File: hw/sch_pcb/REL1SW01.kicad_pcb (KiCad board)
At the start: 2 copper layers, 30 x 40.1 mm, 22 parts, among them J1 HEADER_2x02_PARALLEL, J2 HEADER_2x02_PARALLEL, J3 HEADER_2x06_PARALLEL, J4 HEADER_2x06_PARALLEL, J5 HEADER_2x04_PARALLEL, M1 SROUB3M, M2 SROUB3M, M3 SROUB3M, M4 SROUB3M, T1 IRLML6244, T2 IRLML6244, X1 RELE

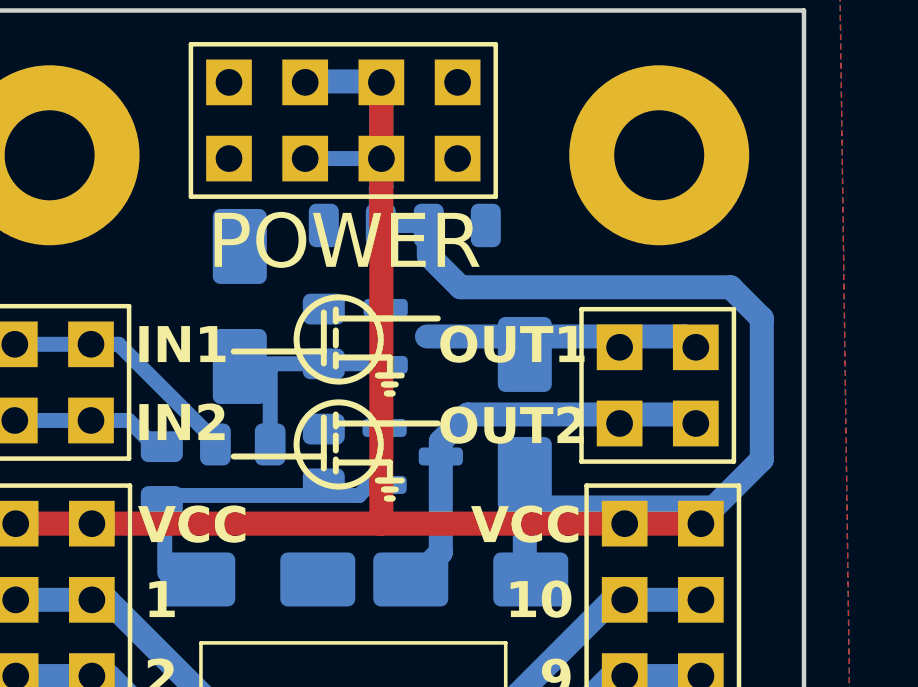
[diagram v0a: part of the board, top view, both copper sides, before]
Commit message: update template
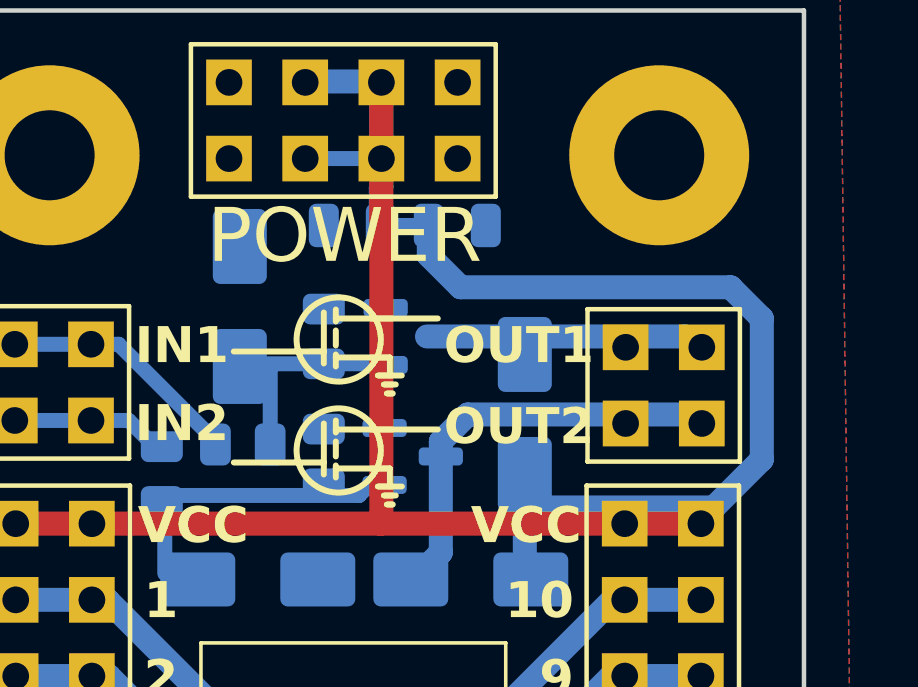
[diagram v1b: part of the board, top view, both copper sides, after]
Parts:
- moved J2 0.20 mm to (158.8, 97.4)
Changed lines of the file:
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@@
   )
   (paper "A4")
+  (title_block
+    (title "REL1SW01B")
+    (date "2024-06-03")
+    (rev "01B")
+    (company "www.mlab.cz")
+    (comment 1 "roman-dvorak <romandvorak@mlab.cz>")
+  )
   (layers
     (0 "F.Cu" signal)
@@
   )
   (footprint "Mlab_Pin_Headers:Straight_2x02" (layer "F.Cu")
-    (at 158.609999 97.43)
+    (at 158.809999 97.43)
     (descr "pin header straight 2x02")
     (tags "pin header straight 2x02")
@@
     )
   )
-  (gr_line (start 147.879999 100) (end 149.679999 100)
-    (stroke (width 0.2) (type default)) (layer "F.SilkS"))
-  (gr_line (start 147.479999 98.5) (end 147.479999 100.2)
-    (stroke (width 0.2) (type default)) (layer "F.SilkS"))
-  (gr_line (start 149.179999 98.7) (end 151.279999 98.7)
+  (gr_line (start 147.879999 100.2) (end 149.679999 100.2)
+    (stroke (width 0.2) (type default)) (layer "F.SilkS"))
+  (gr_line (start 147.479999 98.7) (end 147.479999 100.4)
+    (stroke (width 0.2) (type default)) (layer "F.SilkS"))
+  (gr_line (start 149.179999 98.9) (end 151.279999 98.9)
     (stroke (width 0.2) (type default)) (layer "F.SilkS"))
   (gr_line (start 149.579999 97.7) (end 149.779999 97.7)
     (stroke (width 0.2) (type default)) (layer "F.SilkS"))
-  (gr_line (start 149.679999 100) (end 149.679999 100.6)
+  (gr_line (start 149.679999 100.2) (end 149.679999 100.8)
     (stroke (width 0.2) (type default)) (layer "F.SilkS"))
   (gr_line (start 147.479999 96.3) (end 144.479999 96.3)
@@
   (gr_line (start 147.879999 96.8) (end 147.879999 96.4)
     (stroke (width 0.2) (type default)) (layer "F.SilkS"))
-  (gr_line (start 147.879999 98.7) (end 149.179999 98.7)
+  (gr_line (start 147.879999 98.9) (end 149.179999 98.9)
     (stroke (width 0.2) (type default)) (layer "F.SilkS"))
   (gr_line (start 147.879999 95.2) (end 149.179999 95.2)
     (stroke (width 0.2) (type default)) (layer "F.SilkS"))
-  (gr_line (start 147.879999 98.4) (end 147.879999 98.8)
+  (gr_line (start 147.879999 98.6) (end 147.879999 99)
     (stroke (width 0.2) (type default)) (layer "F.SilkS"))
   (gr_line (start 149.479999 97.4) (end 149.879999 97.4)
     (stroke (width 0.2) (type default)) (layer "F.SilkS"))
-  (gr_circle (center 147.976433 99.4) (end 149.376433 99.5)
+  (gr_circle (center 147.976433 99.6) (end 149.376433 99.7)
     (stroke (width 0.2) (type default)) (fill none) (layer "F.SilkS"))
-  (gr_line (start 147.879999 99.6) (end 147.879999 99.1)
+  (gr_line (start 147.879999 99.8) (end 147.879999 99.3)
     (stroke (width 0.2) (type default)) (layer "F.SilkS"))
   (gr_line (start 149.279999 97.1) (end 150.079999 97.1)
     (stroke (width 0.2) (type default)) (layer "F.SilkS"))
-  (gr_line (start 149.479999 100.9) (end 149.879999 100.9)
+  (gr_line (start 149.479999 101.1) (end 149.879999 101.1)
     (stroke (width 0.2) (type default)) (layer "F.SilkS"))
   (gr_line (start 147.879999 94.9) (end 147.879999 95.3)
@@
   (gr_line (start 149.679999 96.5) (end 149.679999 97.1)
     (stroke (width 0.2) (type default)) (layer "F.SilkS"))
-  (gr_line (start 147.879999 100.3) (end 147.879999 99.9)
-    (stroke (width 0.2) (type default)) (layer "F.SilkS"))
-  (gr_line (start 147.479999 99.8) (end 144.479999 99.8)
+  (gr_line (start 147.879999 100.5) (end 147.879999 100.1)
+    (stroke (width 0.2) (type default)) (layer "F.SilkS"))
+  (gr_line (start 147.479999 100) (end 144.479999 100)
     (stroke (width 0.2) (type default)) (layer "F.SilkS"))
   (gr_circle (center 147.976433 95.9) (end 149.376433 96)
@@
   (gr_line (start 147.879999 96.1) (end 147.879999 95.6)
     (stroke (width 0.2) (type default)) (layer "F.SilkS"))
-  (gr_line (start 149.279999 100.6) (end 150.079999 100.6)
+  (gr_line (start 149.279999 100.8) (end 150.079999 100.8)
     (stroke (width 0.2) (type default)) (layer "F.SilkS"))
   (gr_line (start 149.179999 95.2) (end 151.279999 95.2)
     (stroke (width 0.2) (type default)) (layer "F.SilkS"))
-  (gr_line (start 149.579999 101.2) (end 149.779999 101.2)
+  (gr_line (start 149.579999 101.4) (end 149.779999 101.4)
     (stroke (width 0.2) (type default)) (layer "F.SilkS"))
   (gr_rect (start 133.513999 84.934) (end 163.486 125.066)
@@
     (effects (font (size 1.2 1.2) (thickness 0.2) bold) (justify left bottom))
   )
-  (gr_text "OUT2" (at 151.279999 99.5) (layer "F.SilkS")
+  (gr_text "OUT2" (at 151.479999 99.5) (layer "F.SilkS")
     (effects (font (size 1.2 1.2) (thickness 0.2) bold) (justify left bottom))
   )
@@
     (effects (font (size 1.2 1.2) (thickness 0.2) bold) (justify left bottom))
   )
-  (gr_text "OUT1" (at 151.279999 96.8) (layer "F.SilkS")
-    (effects (font (size 1.2 1.2) (thickness 0.2) bold) (justify left bottom))
-  )
-  (gr_text "POWER" (at 148.176433 93.7) (layer "F.SilkS")
+  (gr_text "OUT1" (at 151.479999 96.8) (layer "F.SilkS")
+    (effects (font (size 1.2 1.2) (thickness 0.2) bold) (justify left bottom))
+  )
+  (gr_text "POWER" (at 148.176433 93.5) (layer "F.SilkS")
     (effects (font (size 1.8 1.8) (thickness 0.2)) (justify bottom))
   )
@@
     (connect_pads (clearance 0.000001))
     (min_thickness 0.2032) (filled_areas_thickness no)
-    (fill (thermal_gap 0.25) (thermal_bridge_width 0.4564))
+    (fill yes (thermal_gap 0.25) (thermal_bridge_width 0.4564))
     (polygon
       (pts
